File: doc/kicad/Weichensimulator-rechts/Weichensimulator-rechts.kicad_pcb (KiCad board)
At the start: 2 copper layers, 38.1 x 38.1 mm, 15 parts, among them J1 Conn_01x02_Male, J2 Power, J3 Conn_01x02_Male, K1 HFD2_005-S-L2-D

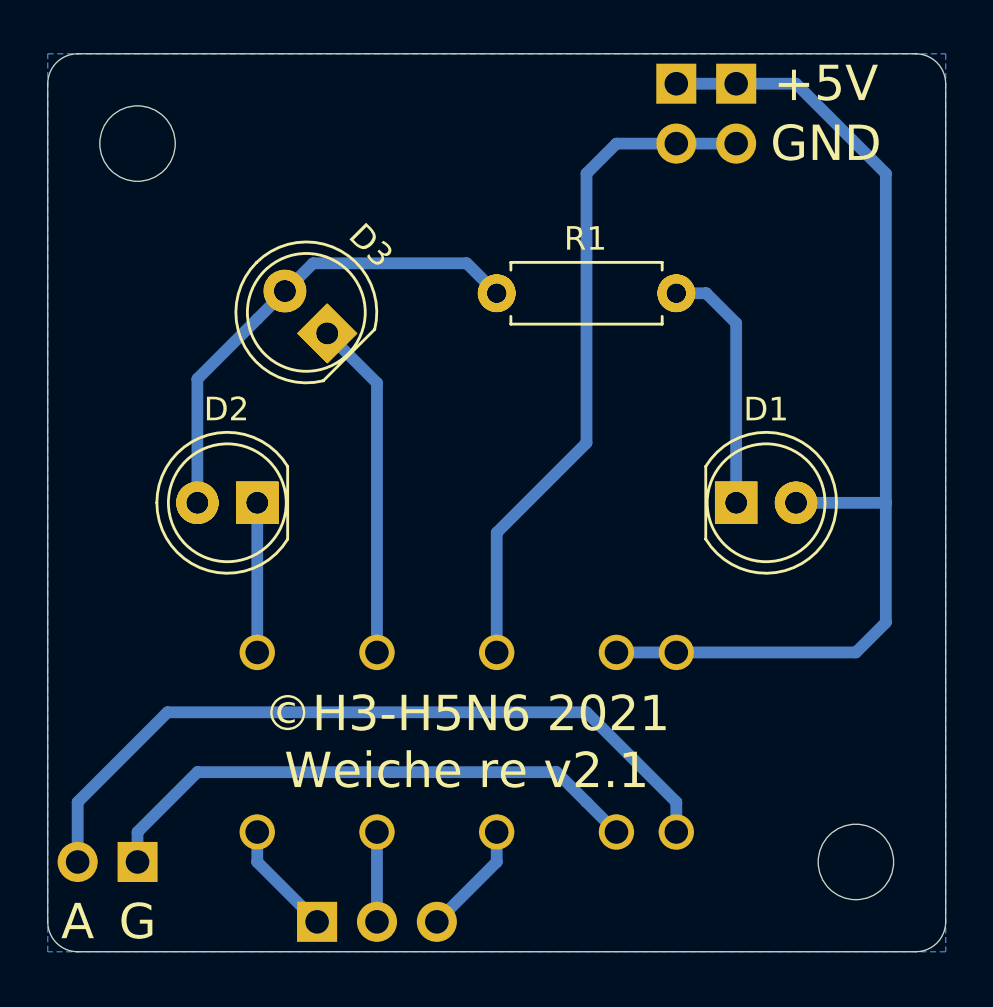
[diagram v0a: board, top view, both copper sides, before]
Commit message: Aufgeräumt
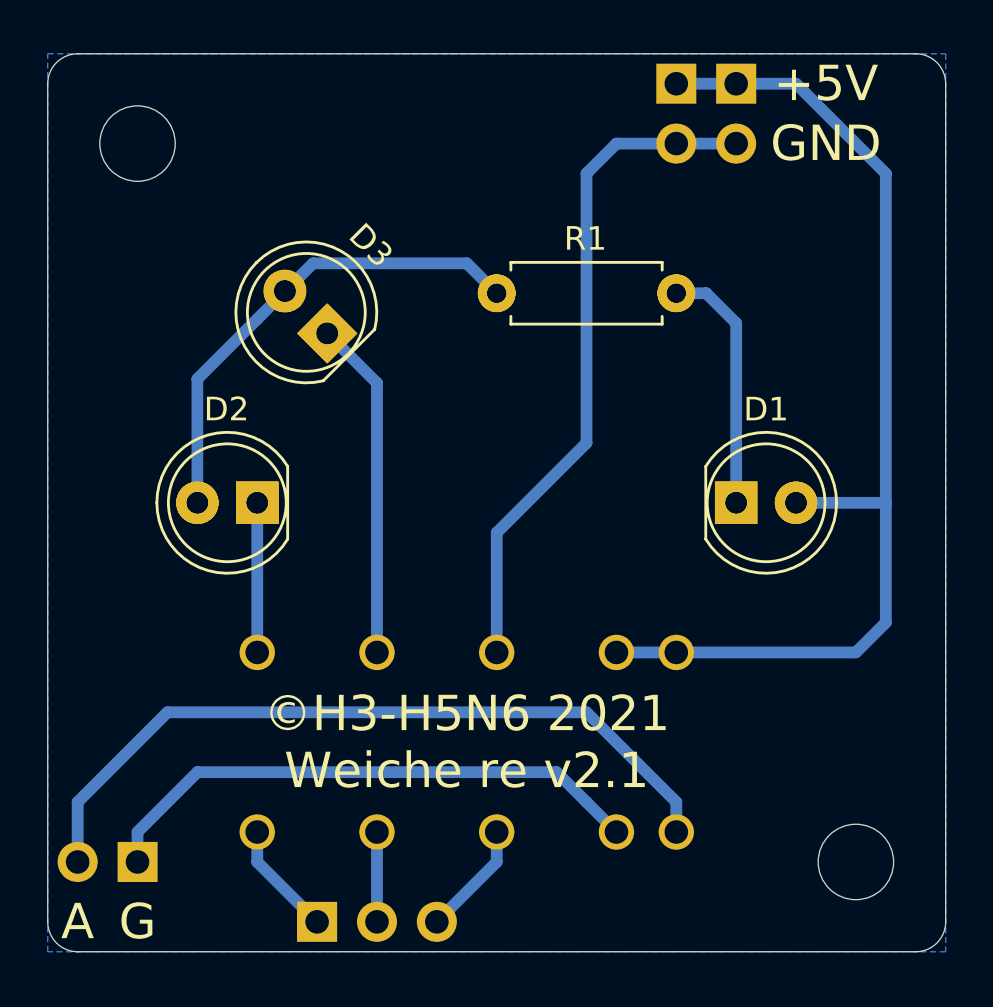
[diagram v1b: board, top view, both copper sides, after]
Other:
- net class Default removed
